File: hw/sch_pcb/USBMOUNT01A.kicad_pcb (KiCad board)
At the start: 2 copper layers, 50 x 20 mm, 18 parts, among them J1 RJ45, P1 USB_C, U1 FT232RL, U2 USBLC6-2SC6

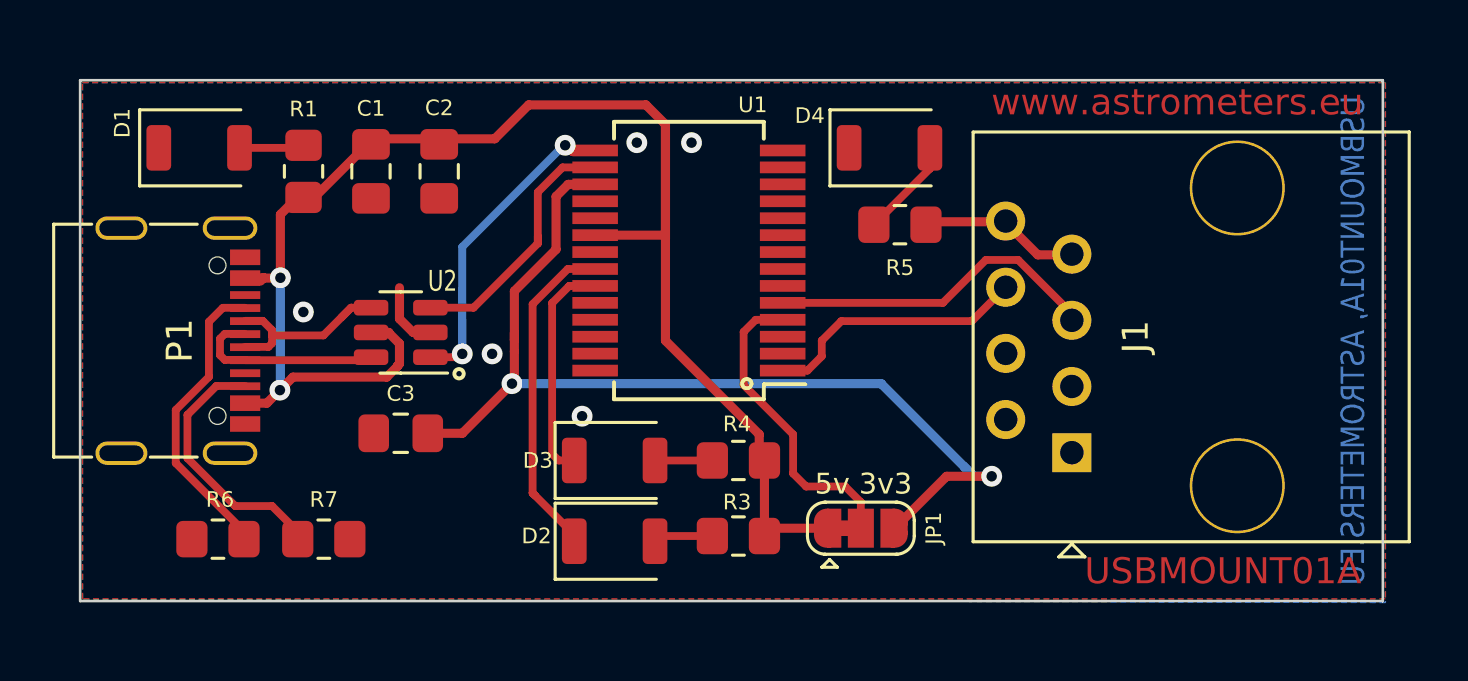
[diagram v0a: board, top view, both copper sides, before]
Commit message: update kicad version
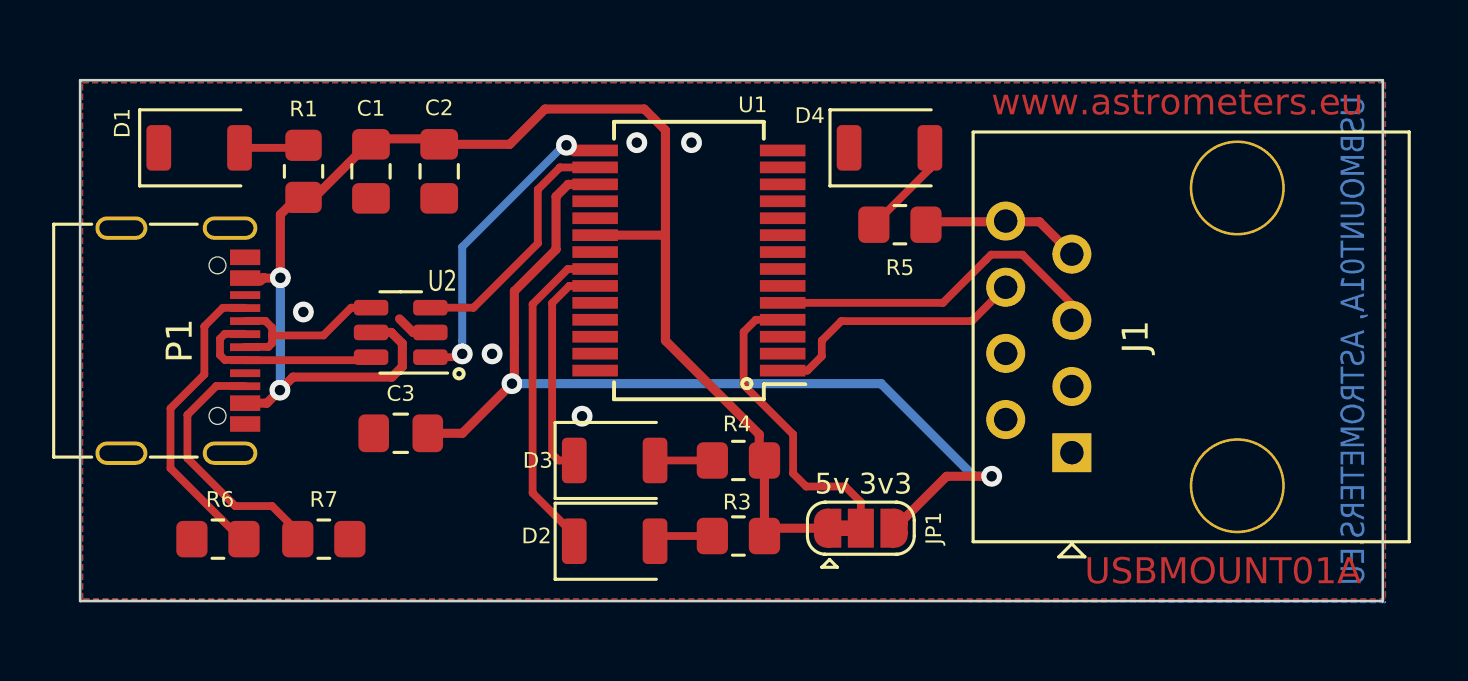
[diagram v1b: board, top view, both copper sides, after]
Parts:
- P1: value USB_C -> USB4105-GF-A
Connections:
- JP1 pad 2: (no net) -> Net-(JP1-Pad2)
- U1 pad 4: (no net) -> Net-(JP1-Pad2)
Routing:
- net Net-(JP1-Pad2): track 0.00 -> 12.0 mm
- net (no net): track 12.0 -> 0.00 mm
- net /D+i: track 14.6 -> 11.7 mm
- net +5V: track 61.7 -> 60.4 mm
- net GND: track 2.60 -> 1.40 mm
- net +3V3: track 39.1 -> 38.0 mm
